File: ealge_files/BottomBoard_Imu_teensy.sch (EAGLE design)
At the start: 96 parts, among them K1 MK20DX256VLH7, K2 MKL04Z32VLC4, T1 MCP1825S, U2 MPU-9250

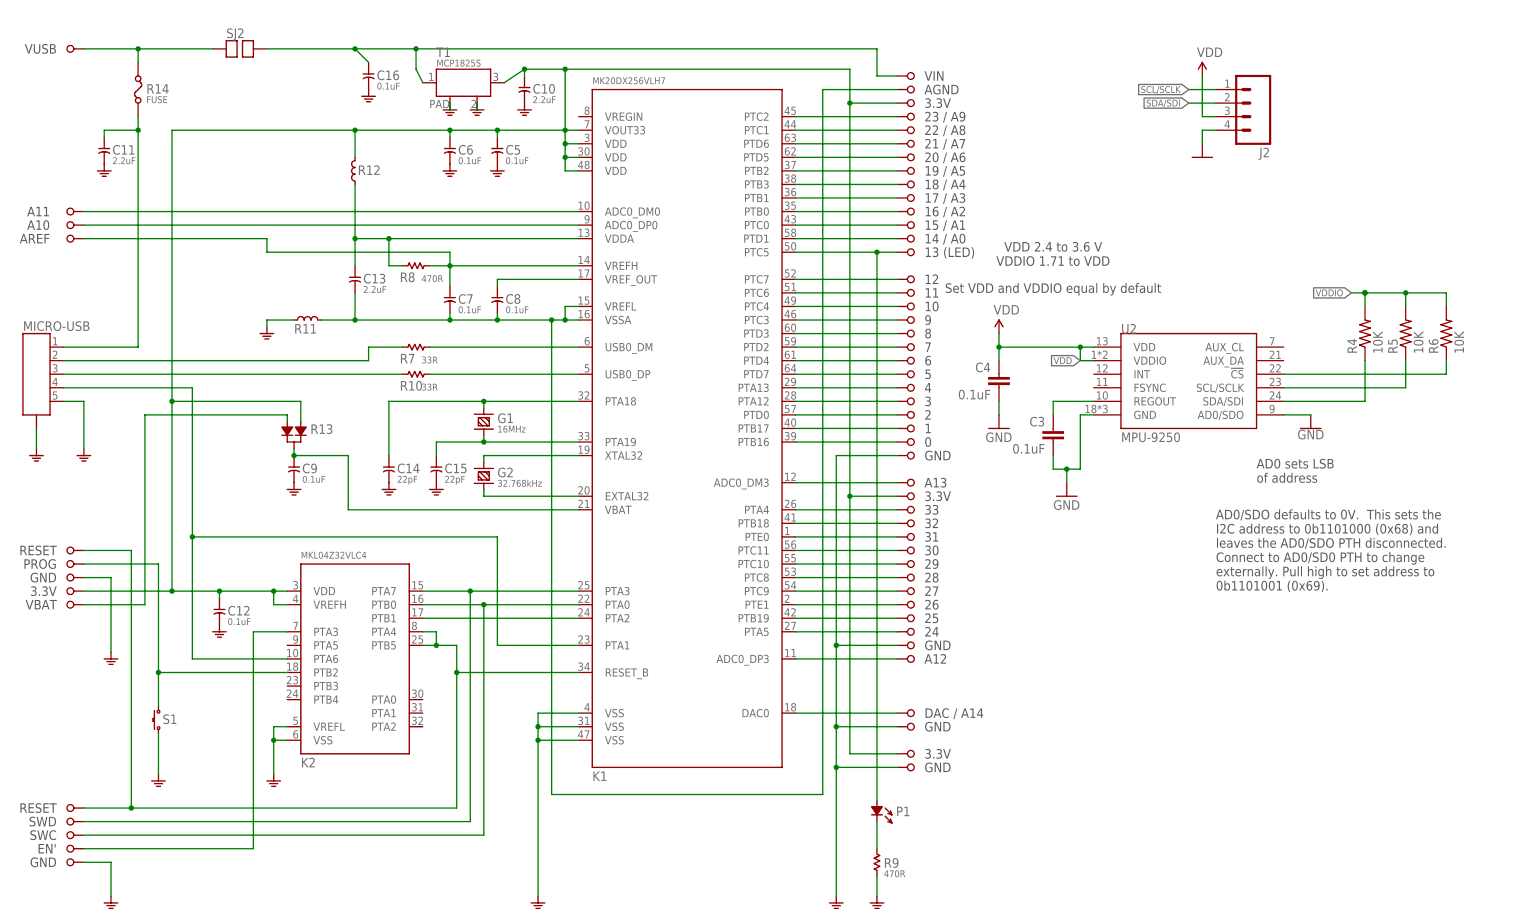
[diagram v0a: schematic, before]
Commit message: completed bottom layer.. and started with nanopi shield
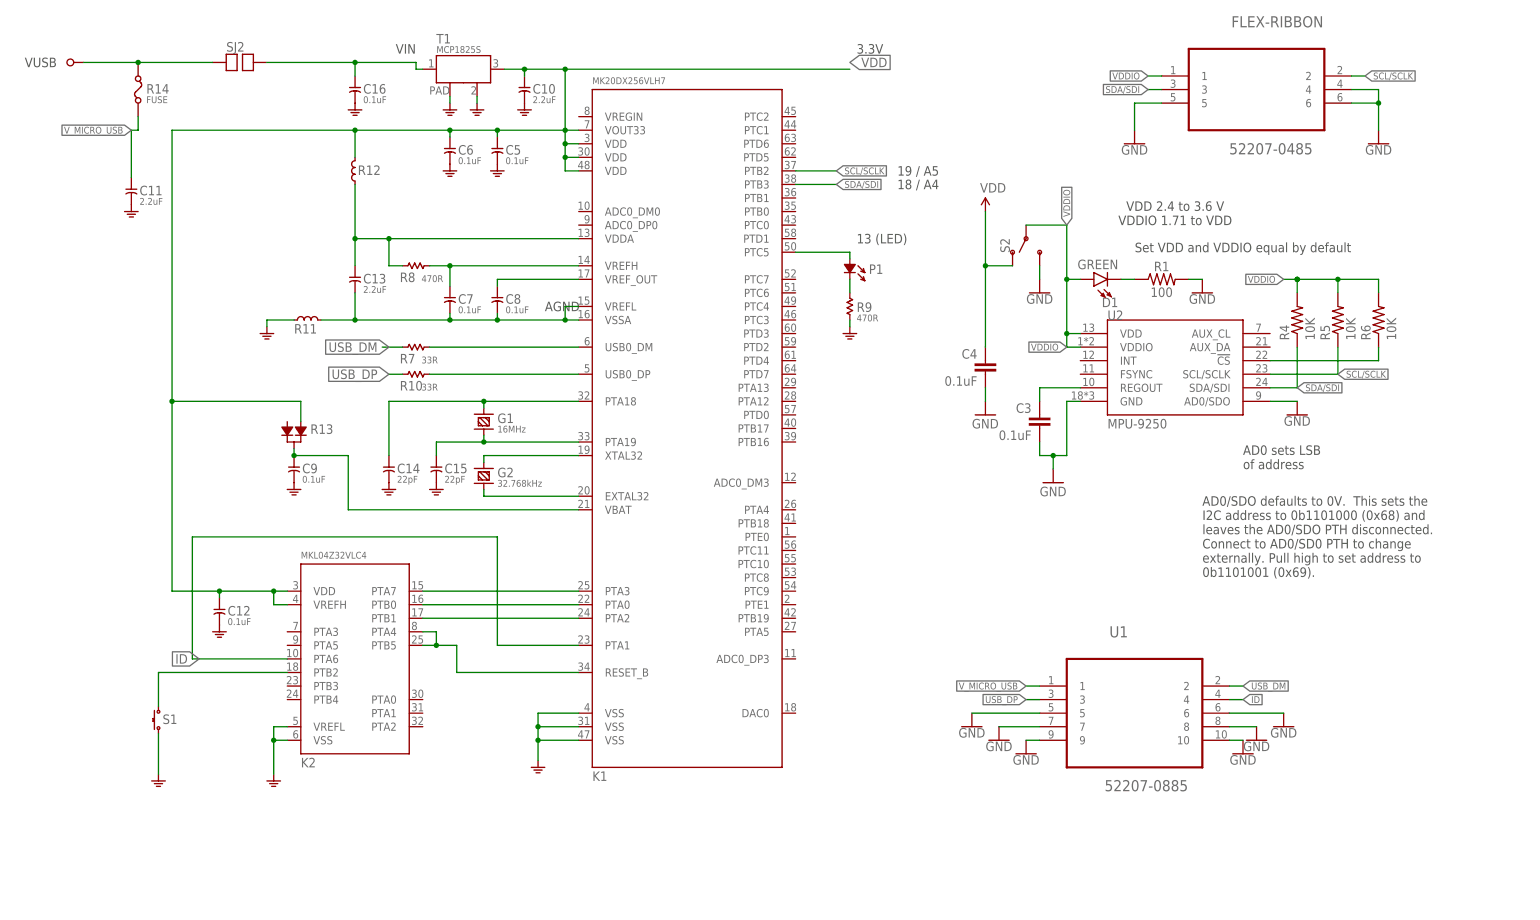
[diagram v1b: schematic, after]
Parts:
- removed J2: (no value), SparkFun-Connectors:M04PTH
- removed MICRO-USB: MINI-USB, t32_ref:MINI-USBMOLEX_0675031230
- removed SX10, SX11, SX12, SX13, SX14, SX15, SX16, SX17, SX18, SX19, SX2, SX20, SX21, SX22, SX23, SX24, SX25, SX26, SX27, SX28, SX29, SX3, SX30, SX31, SX32, SX33, SX34, SX35, SX36, SX37, SX38, SX39, SX4, SX40, SX41, SX42, SX43, SX44, SX45, SX46, SX47, SX48, SX49, SX5, SX50, SX51, SX52, SX53, SX54, SX55, SX56, SX57, SX58, SX59, SX6, SX60, SX7, SX8, SX9: PIN, t32_ref:PIN
- added D1: GREEN, SparkFun-LED:LED-GREEN0603
- added FLEX-RIBBON: 52207-0485, Molex_By_element14_Batch_1:52207-0485
- added R1: 100, SparkFun-Resistors:100OHM-0603-1/4W-5%
- added S2: (no value), SparkFun-Switches:SWITCH-SPDT-SMD-RIGHT-ANGLE
- added U1: 52207-0885, Molex_By_element14_Batch_1:52207-0885
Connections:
- removed net N$12: K1.RESET_B, K2.PTA4, K2.PTB5, SX38.P$1, SX56.P$1
- removed net N$16: MICRO-USB.3, R10.1
- removed net N$17: MICRO-USB.2, R7.1
- removed net N$18: C11.1, MICRO-USB.1, R14.1
- removed net N$19: K1.PTA1, K2.PTA6, MICRO-USB.4
- removed net N$22: K1.PTC1, SX6.P$1
- removed net N$23: K1.PTD6, SX7.P$1
- removed net N$24: K1.PTD5, SX8.P$1
- removed net N$25: K1.PTB2, SX9.P$1
- removed net N$26: K1.PTB3, SX10.P$1
- removed net N$27: K1.PTB1, SX11.P$1
- removed net N$28: K1.PTB0, SX13.P$1
- removed net N$29: K1.PTC0, SX15.P$1
- removed net N$30: K1.PTD1, SX17.P$1
- removed net N$31: K1.PTC5, P1.+, SX18.P$1
- removed net N$32: K1.PTC7, SX19.P$1
- removed net N$33: K1.PTC6, SX20.P$1
- removed net N$34: K1.PTC4, SX21.P$1
- removed net N$35: K1.PTC3, SX22.P$1
- removed net N$36: K1.PTD3, SX23.P$1
- removed net N$37: K1.PTD2, SX24.P$1
- removed net N$38: K1.PTD4, SX25.P$1
- removed net N$39: K1.PTD7, SX26.P$1
- removed net N$40: K1.PTA13, SX27.P$1
- removed net N$41: K1.PTA12, SX28.P$1
- removed net N$42: K1.PTD0, SX29.P$1
- removed net N$43: K1.PTB17, SX30.P$1
- removed net N$44: K1.PTB16, SX31.P$1
- removed net N$45: K1.ADC0_DM3, SX33.P$1
- removed net N$46: K1.PTA4, SX35.P$1
- removed net N$47: K1.PTB18, SX36.P$1
- removed net N$48: K1.PTE0, SX37.P$1
- removed net N$49: K1.PTC11, SX39.P$1
- removed net N$50: K1.PTC10, SX41.P$1
- removed net N$51: K1.PTC8, SX43.P$1
- removed net N$54: K1.DAC0, SX52.P$1
- removed net N$55: K1.ADC0_DP3, SX51.P$1
- removed net N$57: K1.PTA5, SX49.P$1
- removed net N$58: K1.PTB19, SX48.P$1
- removed net N$59: K1.PTE1, SX47.P$1
- removed net N$60: K1.PTC9, SX45.P$1
- removed net N$63: R13.2, SX46.P$1
- removed net N$64: K1.ADC0_DM0, SX12.P$1
- removed net N$65: K1.ADC0_DP0, SX14.P$1
- removed net N$69: C10.1, C12.1, C5.1, C6.1, K1.VDD@3, K1.VDD@30, K1.VDD@48, K1.VOUT33, K2.VDD, K2.VREFH, R12.2, R13.1, SX34.P$1, SX4.P$1, SX44.P$1, SX54.P$1, T1.OUT
- new net ID: K1.PTA1, K2.PTA6, U1.4
- new net N$4: D1.C, R1.1
- new net USB_DM: R7.1, U1.2
- new net USB_DP: R10.1, U1.3
- new net VCC: C4.1, S2.O
- new net V_MICRO_USB: C11.1, R14.1, U1.1
- net GND: now also FLEX-RIBBON.4, FLEX-RIBBON.5, FLEX-RIBBON.6, R1.2, S2.S, U1.10, U1.5, U1.6, U1.7, U1.8, U1.9; no longer J2.4, MICRO-USB.5, MICRO-USB.CASE, SX32.P$1, SX42.P$1, SX50.P$1, SX53.P$1, SX55.P$1, SX60.P$1
- net N$1: now also K1.RESET_B, K2.PTA4, K2.PTB5; no longer K2.PTA3, SX59.P$1
- net N$13: no longer SX16.P$1
- net N$2: no longer SX58.P$1
- net N$21: now also K1.PTC5, P1.+; no longer K1.PTC2, SX5.P$1
- net N$53: no longer SX3.P$1
- net N$61: no longer SX2.P$1
- net N$70: no longer SX57.P$1
- net N$9: no longer SX40.P$1
- net SCL/SCLK: now also FLEX-RIBBON.2, K1.PTB2; no longer J2.1
- net SDA/SDI: now also FLEX-RIBBON.3, K1.PTB3; no longer J2.2
- net VDD: now also C10.1, C12.1, C5.1, C6.1, K1.VDD@3, K1.VDD@30, K1.VDD@48, K1.VOUT33, K2.VDD, K2.VREFH, R12.2, R13.1, T1.OUT; no longer C4.1, J2.3, U2.VDD, U2.VDDIO
- net VDDIO: now also D1.A, FLEX-RIBBON.1, S2.P, U2.VDD, U2.VDDIO
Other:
- note removed: "0"
- note removed: "1"
- note removed: "10"
- note removed: "11"
- note removed: "12"
- note removed: "14 / A0"
- note removed: "15 / A1"
- note removed: "16 / A2"
- note removed: "17 / A3"
- note removed: "2"
- note removed: "20 / A6"
- note removed: "21 / A7"
- note removed: "22 / A8"
- note removed: "23 / A9"
- note removed: "24"
- note removed: "25"
- note removed: "26"
- note removed: "27"
- note removed: "28"
- note removed: "29"
- note removed: "3"
- note removed: "30"
- note removed: "31"
- note removed: "32"
- note removed: "33"
- note removed: "4"
- note removed: "5"
- note removed: "6"
- note removed: "7"
- note removed: "8"
- note removed: "9"
- note removed: "A10"
- note removed: "A11"
- note removed: "A12"
- note removed: "A13"
- note removed: "AREF"
- note removed: "DAC / A14"
- note removed: "EN'"
- note removed: "GND"
- note removed: "PROG"
- note removed: "RESET"
- note removed: "SWC"
- note removed: "SWD"
- note removed: "VBAT"
- moved on the sheet: C11, C16, C3, C4, P1, R4, R5, R6, R9, SJ2, T1, U2
